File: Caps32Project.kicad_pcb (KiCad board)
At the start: 2 copper layers, 22.5 x 35 mm, 37 parts, among them J1 Ph 2.0, J2 Sh 1.0, P1 USB_C_Plug_USB2.0, Q1 AO3401A, SW1 SW_Push, U1 MPU-6050, U2 IP5306, U3 ESP32C3_SuperMini

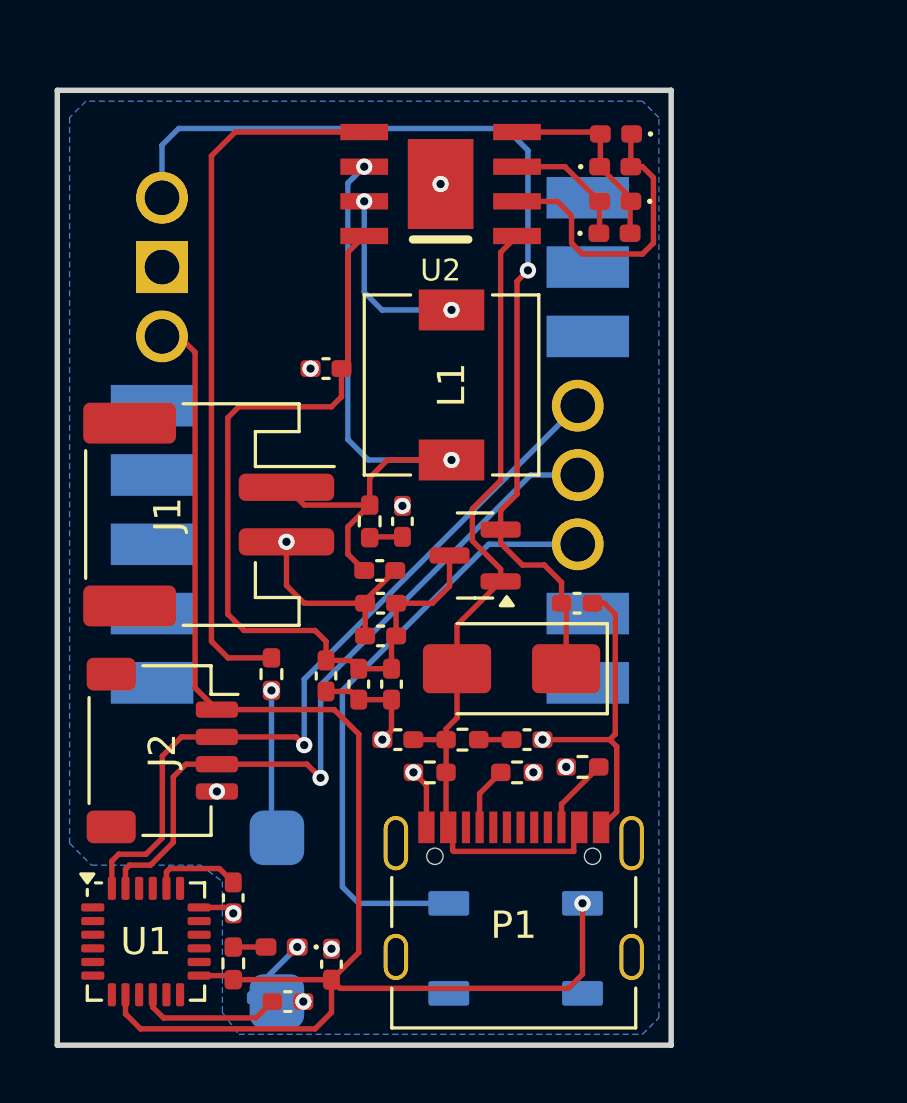
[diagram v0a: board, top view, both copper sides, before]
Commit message: Update Board
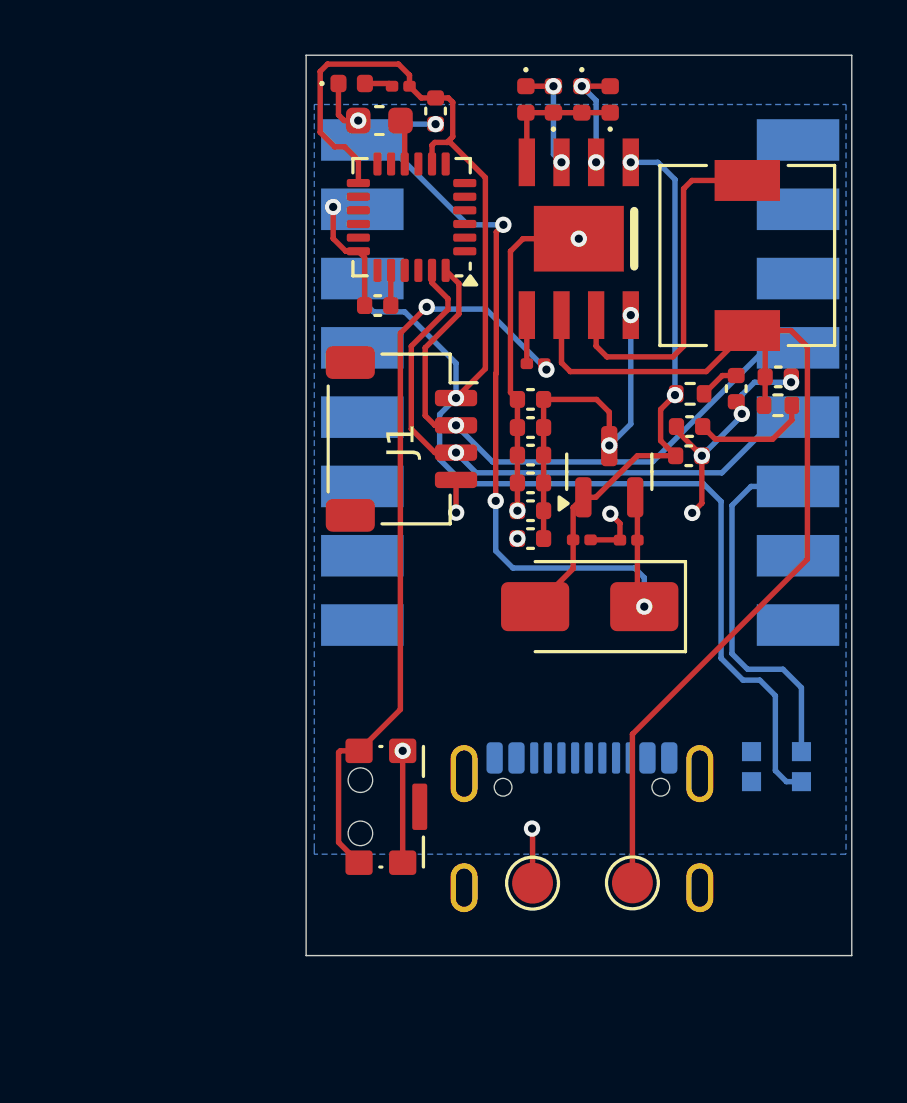
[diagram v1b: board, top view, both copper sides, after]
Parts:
- removed J2: Sh 1.0, Connector_JST:JST_SH_SM04B-SRSS-TB_1x04-1MP_P1.00mm_Horizontal
- removed R6, R7: 5.1K, Resistor_SMD:R_0402_1005Metric_Pad0.72x0.64mm_HandSolder
- added TP1: Bat+, TestPoint:TestPoint_Pad_D1.5mm, F.Cu at (46.6, 54.5)
- added TP2: Bat-, TestPoint:TestPoint_Pad_D1.5mm, F.Cu at (43.0, 54.5)
- C1: value 10uF -> 1.0uF; footprint Capacitor_SMD:C_0402_1005Metric_Pad0.74x0.62mm_HandSolder -> Capacitor_SMD:C_0201_0603Metric
- C10, C11, C12, C2, C7, C8, C9: footprint Capacitor_SMD:C_0402_1005Metric_Pad0.74x0.62mm_HandSolder -> Capacitor_SMD:C_0402_1005Metric
- C13, C6: value 1.0uF -> 10uF; footprint Capacitor_SMD:C_0402_1005Metric_Pad0.74x0.62mm_HandSolder -> Capacitor_SMD:C_0402_1005Metric
- C14: value 10uF -> 1.0uF; footprint Capacitor_SMD:C_0402_1005Metric_Pad0.74x0.62mm_HandSolder -> Capacitor_SMD:C_0402_1005Metric
- C3: value 2.2nF -> 10uF; footprint Capacitor_SMD:C_0402_1005Metric_Pad0.74x0.62mm_HandSolder -> Capacitor_SMD:C_0402_1005Metric
- C4: value 0.1uF -> 2.2nF; footprint Capacitor_SMD:C_0402_1005Metric_Pad0.74x0.62mm_HandSolder -> Capacitor_SMD:C_0603_1608Metric
- C5: value 10uF -> 0.1uF; footprint Capacitor_SMD:C_0402_1005Metric_Pad0.74x0.62mm_HandSolder -> Capacitor_SMD:C_0402_1005Metric
- D1, D4, D5: footprint LED_SMD:LED_0402_1005Metric_Pad0.77x0.64mm_HandSolder -> LED_SMD:LED_0402_1005Metric
- D2: value LED -> SS34; footprint LED_SMD:LED_0402_1005Metric_Pad0.77x0.64mm_HandSolder -> Diode_SMD:D_SMA
- D3: value WS2812B -> LED; footprint LED_SMD:LED_WS2812B_PLCC4_5.0x5.0mm_P3.2mm -> LED_SMD:LED_0402_1005Metric; moved to F.Cu
- D6: value SS34 -> LED; footprint Diode_SMD:D_SMA -> LED_SMD:LED_0402_1005Metric
- D7: value LED -> WS2812B-2020; footprint LED_SMD:LED_0402_1005Metric_Pad0.77x0.64mm_HandSolder -> LED_SMD:LED_WS2812B-2020_PLCC4_2.0x2.0mm; moved to B.Cu
- J1: value Ph 2.0 -> Sh 1.0; footprint Connector_JST:JST_PH_S2B-PH-SM4-TB_1x02-1MP_P2.00mm_Horizontal -> Connector_JST:JST_SH_SM04B-SRSS-TB_1x04-1MP_P1.00mm_Horizontal
- P1: footprint Connector_USB:USB_C_Receptacle_Palconn_UTC16-G -> Connector_USB:USB_C_Receptacle_GCT_USB4105-xx-A_16P_TopMnt_Horizontal; moved to B.Cu
- R1, R4: footprint Resistor_SMD:R_0402_1005Metric_Pad0.72x0.64mm_HandSolder -> Resistor_SMD:R_0201_0603Metric
- R2: value 2R -> 10K; footprint Resistor_SMD:R_0402_1005Metric_Pad0.72x0.64mm_HandSolder -> Resistor_SMD:R_0201_0603Metric
- R3: footprint Resistor_SMD:R_0402_1005Metric_Pad0.72x0.64mm_HandSolder -> Resistor_SMD:R_0402_1005Metric
- R5: value 10K -> 2R; footprint Resistor_SMD:R_0402_1005Metric_Pad0.72x0.64mm_HandSolder -> Resistor_SMD:R_0402_1005Metric
- SW1: footprint Button_Switch_SMD:SW_Push_1TS009xxxx-xxxx-xxxx_6x6x5mm -> Button_Switch_SMD:SW_SPST_CK_KMS2xxGP; moved to F.Cu
- U1: footprint Sensor_Motion:InvenSense_QFN-24_4x4mm_P0.5mm -> Sensor_Motion:InvenSense_QFN-24_4x4mm_P0.5mm_NoMask
- U3: footprint Custom:Supermini_Custom -> Custom:ESP32C3_Supermini_SMD
- moved R1 32.7 mm to (38.1, 25.2), turned to 180 degrees
- moved D1 31.8 mm to (36.3, 25.1), turned to 0 degrees
- moved D3 31.3 mm to (45.8, 25.7), turned to 90 degrees
- moved C4 29.0 mm to (37.4, 26.5), turned to 0 degrees
- moved U1 28.3 mm to (38.5, 30.1), turned to 180 degrees
- moved C3 24.8 mm to (48.7, 38.8), turned to 0 degrees
- moved C6 23.7 mm to (48.7, 37.7), turned to 0 degrees
- moved C14 21.1 mm to (39.4, 26.2)
- moved D6 20.9 mm to (42.7, 25.7), turned to -90 degrees
- moved D7 20.4 mm to (51.9, 50.2)
- moved R5 18.5 mm to (52.0, 36.9), turned to 0 degrees
- moved C2 17.9 mm to (50.4, 36.3), turned to 90 degrees
- moved C7 16.2 mm to (52.0, 35.9)
- moved D2 16.2 mm to (45.1, 44.3), turned to 180 degrees
- moved R4 14.9 mm to (43.1, 35.4), turned to 180 degrees
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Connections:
- C1 pad 1: GND -> +5V
- C1 pad 2: Net-(C1-Pad2) -> GND
- C13 pad 1: +5V -> VCC
- C14 pad 1: VCC -> +3V3
- C2 pad 1: VBUS -> GND
- C2 pad 2: GND -> Net-(C2-Pad2)
- C3 pad 1: GND -> VBUS
- C3 pad 2: Net-(U1-REGOUT) -> GND
- C4 pad 1: Net-(U1-CPOUT) -> GND
- C4 pad 2: GND -> Net-(U1-REGOUT)
- C5 pad 1: GND -> Net-(U1-CPOUT)
- C5 pad 2: Net-(C5-Pad2) -> GND
- C6 pad 1: +3V3 -> GND
- C6 pad 2: GND -> Net-(C6-Pad2)
- D2 pad 1: Net-(D2-K) -> +5V
- D2 pad 2: Net-(D2-A) -> VBUS
- D3 pad 1: +3V3 -> Net-(D3-K)
- D3 pad 2: unconnected-(D3-DOUT-Pad2) -> Net-(D3-A)
- D4 pad 1: Net-(D2-A) -> Net-(D3-A)
- D4 pad 2: Net-(D2-K) -> Net-(D3-K)
- D5 pad 1: Net-(D2-K) -> Net-(D3-K)
- D6 pad 1: +5V -> Net-(D5-A)
- D6 pad 2: VBUS -> Net-(D3-K)
- D7 pad 1: Net-(D5-A) -> unconnected-(D7-DOUT-Pad1)
- D7 pad 2: Net-(D2-K) -> GND
- J1 pad 1: +BATT -> +3V3
- J1 pad 2: GND -> SDA
- P1 pad A5: Net-(P1-CC1) -> unconnected-(P1-CC1-PadA5)
- P1 pad B5: Net-(P1-CC2) -> unconnected-(P1-CC2-PadB5)
- R2 pad 2: Net-(C1-Pad2) -> GND
- R3 pad 1: +BATT -> VBUS
- R3 pad 2: Net-(C5-Pad2) -> Net-(C2-Pad2)
- R5 pad 1: VBUS -> +BATT
- R5 pad 2: GND -> Net-(C6-Pad2)
- U2 pad 2: Net-(D2-A) -> Net-(D3-A)
- U2 pad 4: Net-(D2-K) -> Net-(D3-K)
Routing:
- net Net-(U2-KEY): track 26.2 -> 1.78 mm
- net Net-(R4-Pad1): track 5.49 -> 28.0 mm, vias 1 -> 2
- net VCC: track 31.0 -> 14.1 mm, vias 0 -> 2
- net +BATT: track 24.9 -> 37.1 mm, vias 2 -> 0
- net Net-(D2-A): track 11.2 -> 0.00 mm
- net GND: track 29.7 -> 40.3 mm
- net VBUS: track 31.2 -> 21.3 mm, vias 0 -> 2
- net RGB: track 22.2 -> 13.5 mm
- net Net-(D2-K): track 7.22 -> 0.00 mm
- net +5V: track 36.8 -> 29.6 mm, vias 1 -> 3
- net SDA: track 28.4 -> 22.1 mm
- net Net-(U2-SW): track 6.80 -> 12.9 mm, vias 2 -> 0
- net Net-(D3-K): track 0.00 -> 4.92 mm
- net SCL: track 27.1 -> 22.3 mm
- net Net-(C6-Pad2): track 0.00 -> 4.29 mm
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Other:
- board size 22.5 x 35 mm -> 20 x 33 mm
